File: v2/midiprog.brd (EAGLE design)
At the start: 100 x 80 mm, 56 parts, among them IC1 PIC18F4550_40, IC2 TPIC6B596N, IC3 78L05Z, IC4 TPIC6B596N, Q1 8MHz, Q2 2N2222A, Q3 2N2222A, Q4 2N2222A

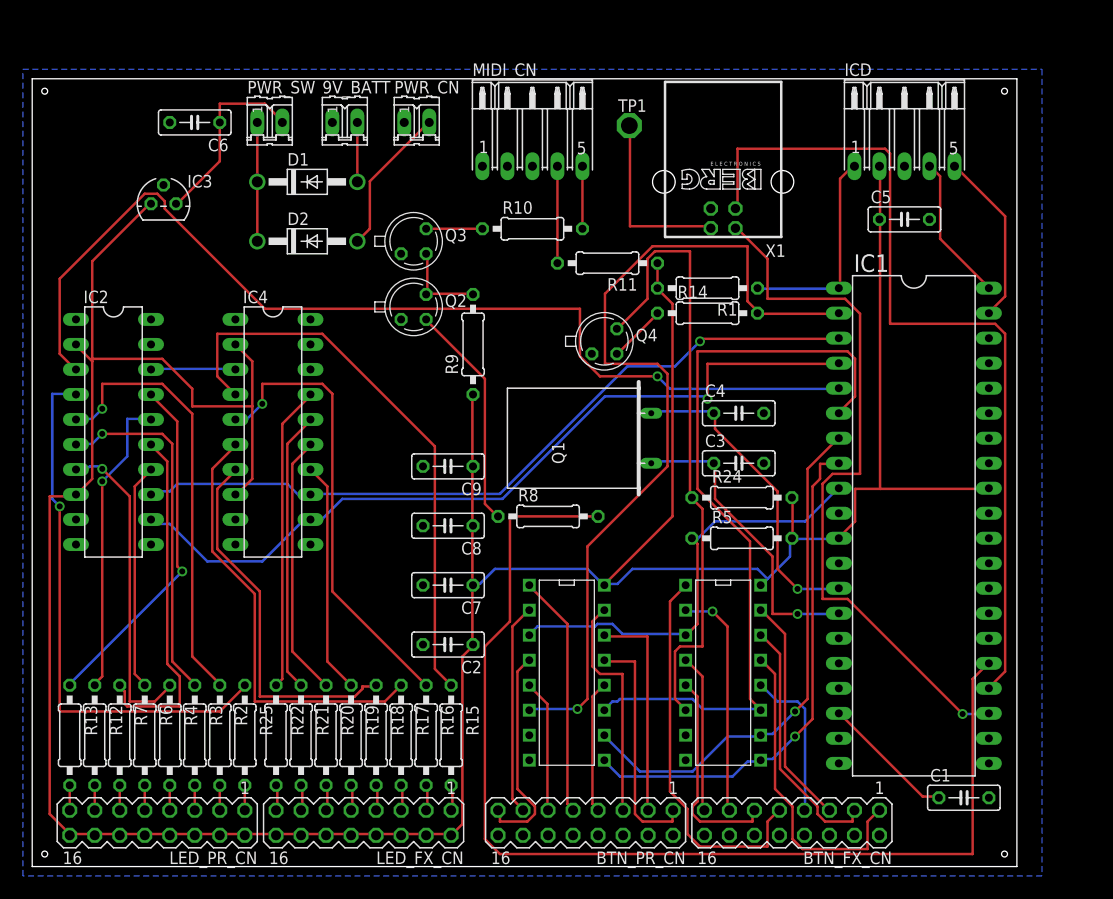
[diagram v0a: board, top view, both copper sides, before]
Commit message: Decent layout; not great.
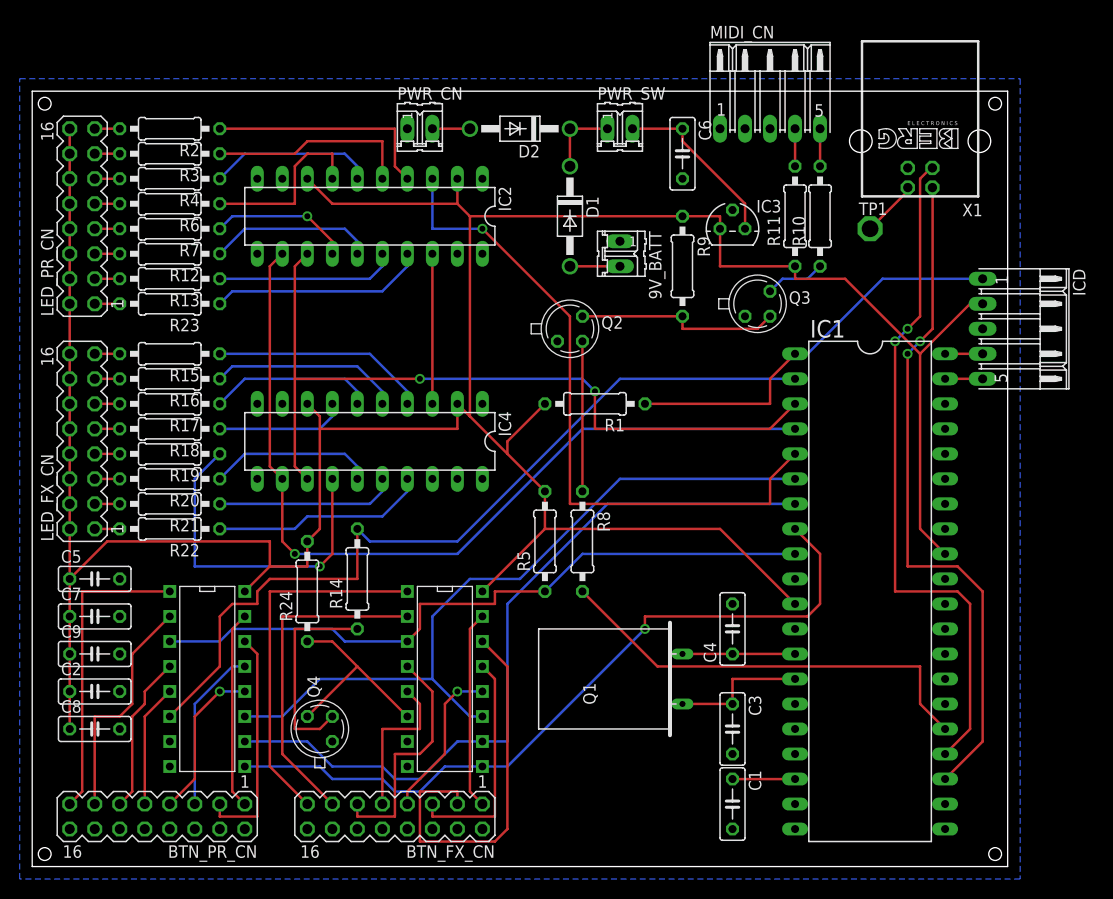
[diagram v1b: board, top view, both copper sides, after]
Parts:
- removed R25: 220, rcl:0207/10
- added R23: 220, rcl:0207/10
- moved C5 90.0 mm to (6.35, 29.2)
- moved LED_PR_CN 62.1 mm to (5.08, 66.0), turned to 90 degrees
- moved R2 61.8 mm to (14.0, 74.9), turned to 180 degrees
- moved R3 59.1 mm to (14.0, 72.4), turned to 180 degrees
- moved IC3 57.8 mm to (71.1, 64.8)
- moved R4 56.5 mm to (14.0, 69.8), turned to 180 degrees
- moved R6 54.0 mm to (14.0, 67.3), turned to 180 degrees
- moved R7 51.7 mm to (14.0, 64.8), turned to 180 degrees
- moved C6 49.6 mm to (66.0, 72.4), turned to 270 degrees
- moved R12 49.5 mm to (14.0, 62.2), turned to 180 degrees
- moved Q4 48.8 mm to (29.2, 14.0), turned to 90 degrees
- moved LED_FX_CN 48.1 mm to (5.08, 43.2), turned to 90 degrees
- moved R15 48.1 mm to (14.0, 52.1), turned to 180 degrees
- moved R13 47.5 mm to (14.0, 59.7), turned to 180 degrees
- moved R24 45.1 mm to (27.9, 27.9), turned to 90 degrees
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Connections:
- net BFX2 renamed N$63
- net BFX4 renamed N$61
- net BFX7 renamed N$49
- net BPR2 renamed N$57
- net BPR4 renamed N$55
- net BPR7 renamed N$51
- removed net BFX1: BTN_FX_CN.1, U$2.13
- removed net BFX3: BTN_FX_CN.5, U$2.15
- removed net BFX5: BTN_FX_CN.9, U$2.1
- removed net BFX6: BTN_FX_CN.11, U$2.5
- removed net BFX8: BTN_FX_CN.15, U$2.4
- removed net BPR1: BTN_PR_CN.1, U$1.13
- removed net BPR3: BTN_PR_CN.5, U$1.15
- removed net BPR5: BTN_PR_CN.9, U$1.1
- removed net BPR6: BTN_PR_CN.11, U$1.5
- removed net BPR8: BTN_PR_CN.15, U$1.4
- removed net N$19 (its old number): LED_FX_CN.9, R19.2
- removed net N$20 (its old number): LED_FX_CN.7, R18.2
- removed net N$21 (its old number): LED_FX_CN.5, R17.2
- removed net N$22 (its old number): LED_FX_CN.3, R16.2
- removed net N$23 (its old number): LED_FX_CN.1, R15.2
- new net N$10: LED_FX_CN.11, R17.2
- new net N$13: LED_FX_CN.5, R20.2
- new net N$14: LED_FX_CN.3, R21.2
- new net N$15: LED_FX_CN.1, R22.2
- new net N$3: LED_FX_CN.13, R16.2
- new net N$46: BTN_FX_CN.9, U$2.5
- new net N$47: BTN_PR_CN.9, U$1.5
- new net N$48: BTN_FX_CN.11, U$2.4
- new net N$50: BTN_PR_CN.11, U$1.4
- new net N$52: BTN_PR_CN.15, U$1.1
- new net N$56: BTN_PR_CN.5, U$1.13
- new net N$58: BTN_PR_CN.1, U$1.15
- new net N$60: BTN_FX_CN.15, U$2.1
- new net N$62: BTN_FX_CN.5, U$2.13
- new net N$64: BTN_FX_CN.1, U$2.15
- net N$11: now also LED_FX_CN.9, R18.2; no longer LED_FX_CN.13, R21.2
- net N$12: now also LED_FX_CN.7, R19.2; no longer LED_FX_CN.11, R20.2
- net N$2: now also R15.2; no longer R22.2
- net N$24: now also R3.2; no longer R12.2
- net N$27: now also R4.2; no longer R7.2
- net N$30: now also R7.2; no longer R4.2
- net N$32: now also R12.2; no longer R3.2
- net N$36: now also R13.2; no longer R2.2
- net N$37: now also R23.2; no longer R25.2
- net N$38: now also IC2.4, R2.1; no longer IC2.17, R13.1
- net N$39: now also IC2.5, R3.1; no longer IC2.16, R12.1
- net N$40: now also IC2.6, R4.1; no longer IC2.15, R7.1
- net N$41: now also IC2.7; no longer IC2.14
- net N$42: now also IC2.14, R7.1; no longer IC2.7, R4.1
- net N$43: now also IC2.15, R12.1; no longer IC2.6, R3.1
- net N$44: now also IC2.16, R13.1; no longer IC2.5, R2.1
- net N$45: now also IC2.17, R23.1; no longer IC2.4, R25.1
- net N$6: now also R2.2; no longer R13.2
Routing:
- net MIDI_TX: track 113.0 -> 44.8 mm
- net N$54: track 63.2 -> 20.5 mm
- net BFX5: track 39.5 -> 0.00 mm
- net N$60: track 0.00 -> 37.1 mm
- net N$19: track 58.7 -> 21.9 mm
- net SHIFTREG_D: track 104.1 -> 68.2 mm
- net N$45: track 55.0 -> 21.9 mm, vias 1 -> 0
- net BFX1: track 32.0 -> 0.00 mm
- net N$52: track 0.00 -> 31.0 mm
- net N$21: track 44.4 -> 16.8 mm
- net N$20: track 46.5 -> 19.4 mm, vias 1 -> 0
- net N$44: track 44.8 -> 18.3 mm, vias 1 -> 0
- net BTN_IN: track 44.5 -> 70.5 mm
- net N$22: track 38.0 -> 13.2 mm
- net BPR5: track 24.7 -> 0.00 mm
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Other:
- board size 100 x 80 mm -> 99.1 x 78.7 mm
